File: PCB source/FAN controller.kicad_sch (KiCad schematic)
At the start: 9 parts, among them M1 Fan, Q4 AO3400A

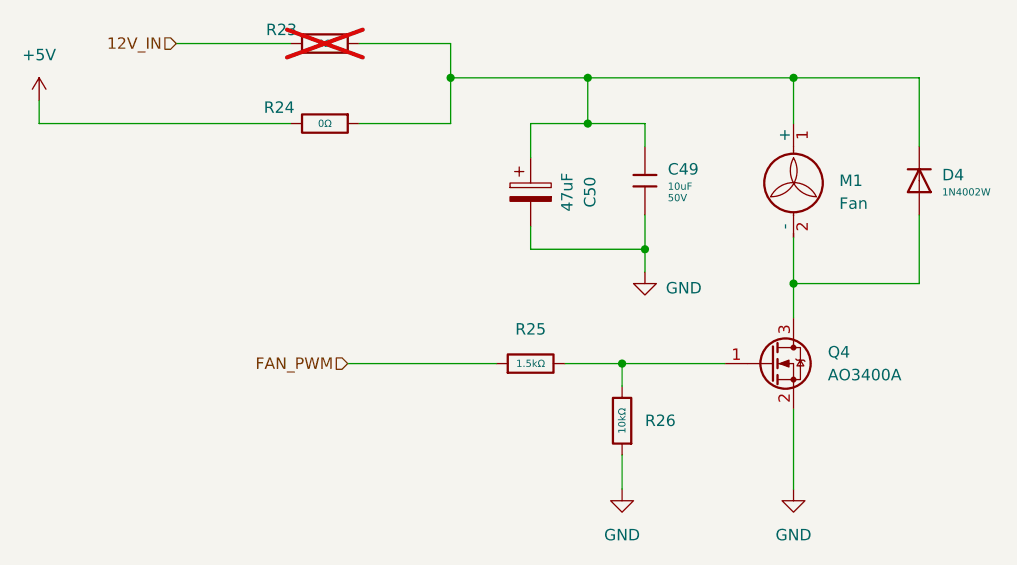
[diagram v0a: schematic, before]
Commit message: Fix schematic
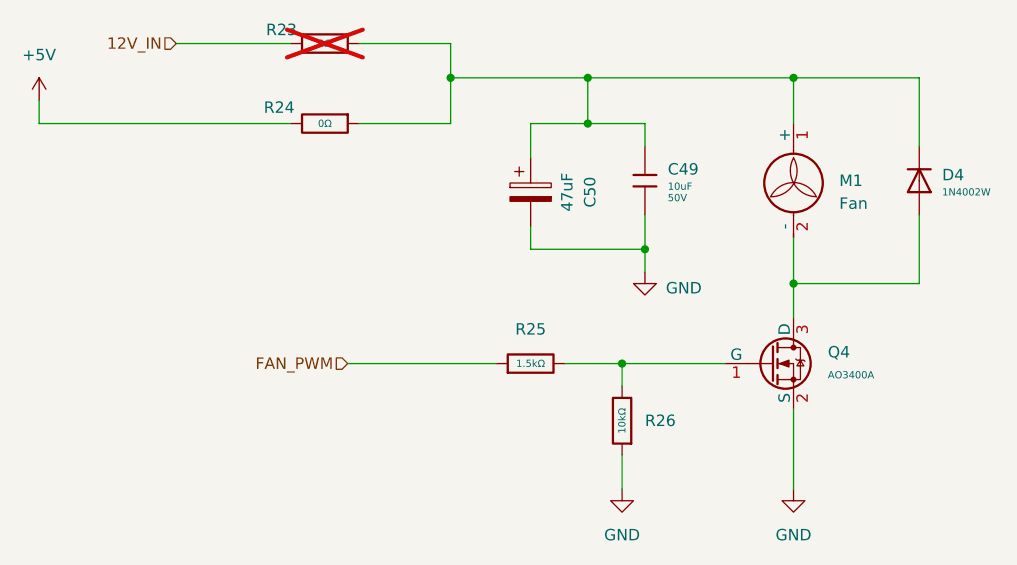
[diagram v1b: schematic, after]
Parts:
- removed Q4: AO3400A, Package_TO_SOT_SMD:SOT-23, symbol Transistor_FET:AO3400A
- added Q4: AO3400A, PCM_JLCPCB:Q_SOT-23, symbol PCM_JLCPCB-Transistors:NMOS,AO3400A
- C49: Price 0.031USD -> 0.035USD; Stock 4852625 -> 821695
- D4: Stock 26897 -> 26535
- R23, R24: Stock 5514860 -> 6249348
- R25: Stock 778464 -> 1074828
- R26: Stock 6666349 -> 13746052
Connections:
- net GND: now also Q4.2 (S)
- net at R25.2, R26.2: now also Q4.1 (G)
- net at D4.2, M1.2 (-): now also Q4.3 (D)
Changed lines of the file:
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@@
 (kicad_sch
-	(version 20231120)
+	(version 20250114)
 	(generator "eeschema")
-	(generator_version "8.0")
+	(generator_version "9.0")
 	(paper "A4")
 	(title_block
@@
 		(shape input)
 		(at 102.87 80.01 180)
-		(fields_autoplaced yes)
 		(effects
 			(font
@@
 		(shape input)
 		(at 121.92 115.57 180)
-		(fields_autoplaced yes)
 		(effects
 			(font
@@
 			)
 		)
-		(property "Stock" "5514860"
+		(property "Stock" "6249348"
 			(at 119.38 80.01 0)
 			(effects
@@
 				(path "/3103c9de-f1ba-4d51-8bfc-798df1c75e2f/ddd125ab-d3f0-4627-8bf0-c5c0a9168cb7"
 					(reference "R23")
-					(unit 1)
-				)
-			)
-		)
-	)
-	(symbol
-		(lib_id "Transistor_FET:AO3400A")
-		(at 168.91 115.57 0)
-		(unit 1)
-		(exclude_from_sim no)
-		(in_bom yes)
-		(on_board yes)
-		(dnp no)
-		(fields_autoplaced yes)
-		(property "Reference" "Q4"
-			(at 175.26 114.3 0)
-			(effects
-				(font
-					(size 1.27 1.27)
-				)
-				(justify left)
-			)
-		)
-		(property "Value" "AO3400A"
-			(at 175.26 116.84 0)
-			(effects
-				(font
-					(size 1.27 1.27)
-				)
-				(justify left)
-			)
-		)
-		(property "Footprint" "Package_TO_SOT_SMD:SOT-23"
-			(at 173.99 117.475 0)
-			(effects
-				(font
-					(size 1.27 1.27)
-					(italic yes)
-				)
-				(justify left)
-				(hide yes)
-			)
-		)
-		(property "Datasheet" "http://www.aosmd.com/pdfs/datasheet/AO3400A.pdf"
-			(at 173.99 119.38 0)
-			(effects
-				(font
-					(size 1.27 1.27)
-				)
-				(justify left)
-				(hide yes)
-			)
-		)
-		(property "Description" "30V Vds, 5.7A Id, N-Channel MOSFET, SOT-23"
-			(at 168.91 115.57 0)
-			(effects
-				(font
-					(size 1.27 1.27)
-				)
-				(hide yes)
-			)
-		)
-		(pin "2"
-		)
-		(pin "1"
-		)
-		(pin "3"
-		)
-		(instances
-			(project ""
-				(path "/3103c9de-f1ba-4d51-8bfc-798df1c75e2f/ddd125ab-d3f0-4627-8bf0-c5c0a9168cb7"
-					(reference "Q4")
 					(unit 1)
 				)
@@
 			)
 		)
-		(property "Stock" "778464"
+		(property "Stock" "1074828"
 			(at 142.24 115.57 0)
 			(effects
@@
 			)
 		)
-		(property "Stock" "4852625"
+		(property "Stock" "821695"
 			(at 154.94 95.25 0)
 			(effects
@@
 			)
 		)
-		(property "Price" "0.031USD"
+		(property "Price" "0.035USD"
 			(at 154.94 95.25 0)
 			(effects
@@
 			)
 		)
-		(property "Stock" "6666349"
+		(property "Stock" "13746052"
 			(at 152.4 121.92 0)
 			(effects
@@
 			)
 		)
-		(property "Stock" "26897"
+		(property "Stock" "26535"
 			(at 185.42 95.25 0)
 			(effects
@@
 			)
 		)
-		(property "Stock" "5514860"
+		(property "Stock" "6249348"
 			(at 119.38 88.9 0)
 			(effects
@@
 					(unit 1)
 				)
+			)
+		)
+	)
+	(symbol
+		(lib_id "PCM_JLCPCB-Transistors:NMOS,AO3400A")
+		(at 168.91 115.57 0)
+		(unit 1)
+		(exclude_from_sim no)
+		(in_bom yes)
+		(on_board yes)
+		(dnp no)
+		(fields_autoplaced yes)
+		(property "Reference" "Q4"
+			(at 175.26 114.2999 0)
+			(effects
+				(font
+					(size 1.27 1.27)
+				)
+				(justify left)
+			)
+		)
+		(property "Value" "AO3400A"
+			(at 175.26 116.84 0)
+			(effects
+				(font
+					(size 0.8 0.8)
+				)
+				(justify left)
+			)
+		)
+		(property "Footprint" "PCM_JLCPCB:Q_SOT-23"
+			(at 167.132 115.57 90)
+			(effects
+				(font
+					(size 1.27 1.27)
+				)
+				(hide yes)
+			)
+		)
+		(property "Datasheet" "https://www.lcsc.com/datasheet/lcsc_datasheet_1811081213_Alpha---Omega-Semicon-AO3400A_C20917.pdf"
+			(at 168.91 115.57 0)
+			(effects
+				(font
+					(size 1.27 1.27)
+				)
+				(hide yes)
+			)
+		)
+		(property "Description" "30V 5.7A 26.5mΩ@10V,5.7A 1.4W 1.5V@250uA 1 N-Channel SOT-23-3L MOSFETs ROHS"
+			(at 168.91 115.57 0)
+			(effects
+				(font
+					(size 1.27 1.27)
+				)
+				(hide yes)
+			)
+		)
+		(property "LCSC" "C20917"
+			(at 168.91 115.57 0)
+			(effects
+				(font
+					(size 1.27 1.27)
+				)
+				(hide yes)
+			)
+		)
+		(property "Stock" "670221"
+			(at 168.91 115.57 0)
+			(effects
+				(font
+					(size 1.27 1.27)
+				)
+				(hide yes)
+			)
+		)
+		(property "Price" "0.088USD"
+			(at 168.91 115.57 0)
+			(effects
+				(font
+					(size 1.27 1.27)
+				)
+				(hide yes)
+			)
+		)
+		(property "Process" "SMT"
+			(at 168.91 115.57 0)
+			(effects
+				(font
+					(size 1.27 1.27)
+				)
+				(hide yes)
+			)
+		)
+		(property "Minimum Qty" "5"
+			(at 168.91 115.57 0)
+			(effects
+				(font
+					(size 1.27 1.27)
+				)
+				(hide yes)
+			)
+		)
+		(property "Attrition Qty" "4"
+			(at 168.91 115.57 0)
+			(effects
+				(font
+					(size 1.27 1.27)
+				)
+				(hide yes)
+			)
+		)
+		(property "Class" "Basic Component"
+			(at 168.91 115.57 0)
+			(effects
+				(font
+					(size 1.27 1.27)
+				)
+				(hide yes)
+			)
+		)
+		(property "Category" "Transistors,MOSFETs"
+			(at 168.91 115.57 0)
+			(effects
+				(font
+					(size 1.27 1.27)
+				)
+				(hide yes)
+			)
+		)
+		(property "Manufacturer" "Alpha & Omega Semicon"
+			(at 168.91 115.57 0)
+			(effects
+				(font
+					(size 1.27 1.27)
+				)
+				(hide yes)
+			)
+		)
+		(property "Part" "AO3400A"
+			(at 168.91 115.57 0)
+			(effects
+				(font
+					(size 1.27 1.27)
+				)
+				(hide yes)
+			)
+		)
+		(property "Continuous Drain Current (Id)" "5.7A"
+			(at 168.91 115.57 0)
+			(effects
+				(font
+					(size 1.27 1.27)
+				)
+				(hide yes)
+			)
+		)
+		(property "Input Capacitance (Ciss@Vds)" "630pF@15V"
+			(at 168.91 115.57 0)
+			(effects
+				(font
+					(size 1.27 1.27)
+				)
+				(hide yes)
+			)
+		)
+		(property "Operating Temperature" "-55°C~+150°C@(Tj)"
+			(at 168.91 115.57 0)
+			(effects
+				(font
+					(size 1.27 1.27)
+				)
+				(hide yes)
+			)
+		)
+		(property "Type" "1 N-channel"
+			(at 168.91 115.57 0)
+			(effects
+				(font
+					(size 1.27 1.27)
+				)
+				(hide yes)
+			)
+		)
+		(property "Drain Source Voltage (Vdss)" "30V"
+			(at 168.91 115.57 0)
+			(effects
+				(font
+					(size 1.27 1.27)
+				)
+				(hide yes)
+			)
+		)
+		(property "Power Dissipation (Pd)" "1.4W"
+			(at 168.91 115.57 0)
+			(effects
+				(font
+					(size 1.27 1.27)
+				)
+				(hide yes)
+			)
+		)
+		(property "Gate Threshold Voltage (Vgs(th)@Id)" "1.5V@250uA"
+			(at 168.91 115.57 0)
+			(effects
+				(font
+					(size 1.27 1.27)
+				)
+				(hide yes)
+			)
+		)
+		(property "Drain Source On Resistance (RDS(on)@Vgs,Id)" "26.5mΩ@10V,5.7A"
+			(at 168.91 115.57 0)
+			(effects
+				(font
+					(size 1.27 1.27)
+				)
+				(hide yes)
+			)
+		)
+		(property "Total Gate Charge (Qg@Vgs)" "7nC@4.5V"
+			(at 168.91 115.57 0)
+			(effects
+				(font
+					(size 1.27 1.27)
+				)
+				(hide yes)
+			)
+		)
+		(pin "1"
+		)
+		(pin "3"
+		)
+		(pin "2"
+		)
+		(instances
+			(project ""
+				(path "/3103c9de-f1ba-4d51-8bfc-798df1c75e2f/ddd125ab-d3f0-4627-8bf0-c5c0a9168cb7"
+					(reference "Q4")
+					(unit 1)
+				)
